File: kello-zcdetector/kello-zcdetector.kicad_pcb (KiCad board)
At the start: 2 copper layers, 8 parts, among them J1 Conn_01x02_Male, J2 Conn_01x02_Male, U1 LTV-817S

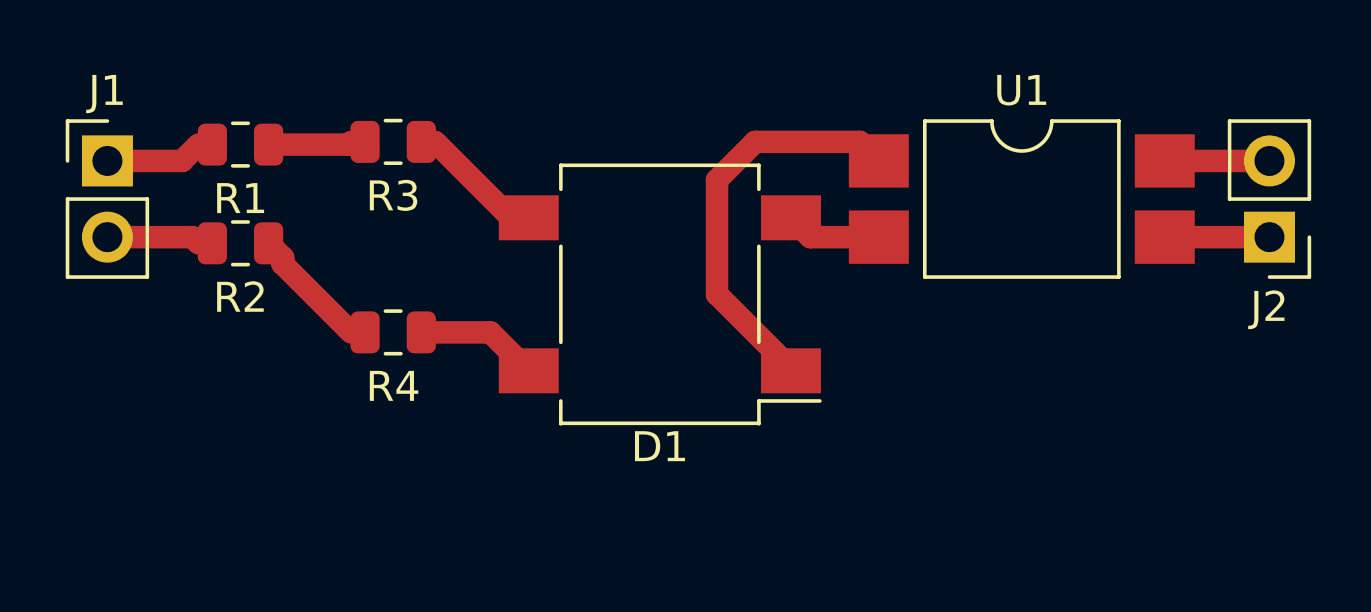
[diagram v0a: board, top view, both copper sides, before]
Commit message: joo
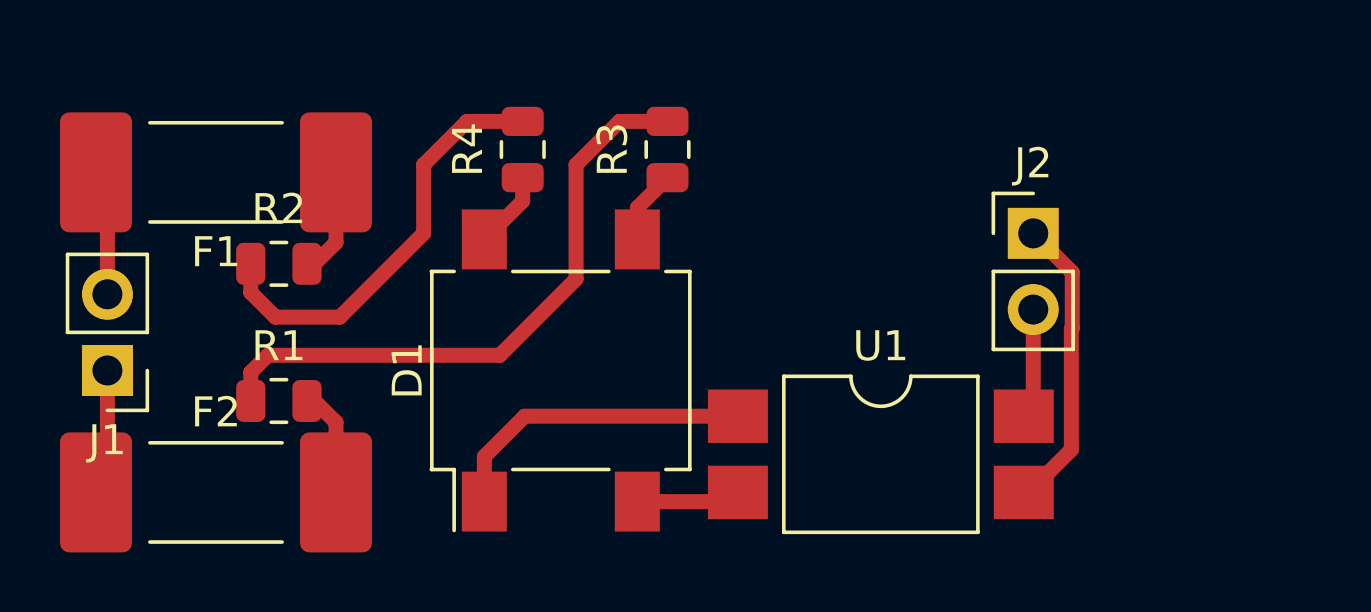
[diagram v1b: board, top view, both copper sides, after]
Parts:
- added F1: Fuse, Fuse:Fuse_10mmx3mm, F.Cu at (17.6, 14.4)
- added F2: Fuse, Fuse:Fuse_10mmx3mm, F.Cu at (17.6, 25.0)
- moved U1 9.72 mm to (39.8, 23.7)
- moved R3 9.15 mm to (32.6, 13.6), turned to 90 degrees
- moved R1 8.64 mm to (19.7, 22.0), turned to 0 degrees
- moved J2 7.88 mm to (44.8, 16.4), turned to 0 degrees
- moved R4 7.47 mm to (27.8, 13.6), turned to 90 degrees
- moved J1 6.98 mm to (14.0, 21.0), turned to 180 degrees
- moved D1 4.17 mm to (29.1, 21.0), turned to 90 degrees
- moved R2 1.45 mm to (19.7, 17.4), turned to 0 degrees
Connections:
- J1 pad 1: Net-(J1-Pad1) -> Net-(F2-Pad1)
- J1 pad 2: Net-(J1-Pad2) -> Net-(F1-Pad2)
- R1 pad 2: Net-(J1-Pad1) -> Net-(F2-Pad2)
- R2 pad 2: Net-(J1-Pad2) -> Net-(F1-Pad1)
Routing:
- net Net-(R1-Pad1): track 2.33 -> 20.3 mm
- net Net-(R2-Pad1): track 4.13 -> 14.1 mm
- net Net-(J2-Pad1): track 3.49 -> 9.94 mm
- net Net-(F2-Pad1): track 0.00 -> 4.14 mm
- net Net-(F1-Pad2): track 0.00 -> 4.14 mm
- net Net-(F2-Pad2): track 0.00 -> 3.70 mm
- net Net-(F1-Pad1): track 0.00 -> 3.70 mm
- net Net-(J1-Pad1): track 3.26 -> 0.00 mm
- net Net-(J1-Pad2): track 3.12 -> 0.00 mm
- net Net-(D1-Pad1): track 13.6 -> 10.5 mm
- net Net-(D1-Pad3): track 4.17 -> 2.48 mm
- net Net-(D1-Pad4): track 3.65 -> 2.59 mm
